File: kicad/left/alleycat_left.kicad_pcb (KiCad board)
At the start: 2 copper layers, 134 x 128 mm, 116 parts, among them J1 Conn_01x04_Male, J2 USB_C_Receptacle_USB2.0, SW1 SW_Push, SW2 RotaryEncoder_Switch, U1 nRF52840_holyiot_18010, U2 TP4056, U3 DW01A, U4 FS8205, U5 SRV05-4, U6 XC6206PxxxMR

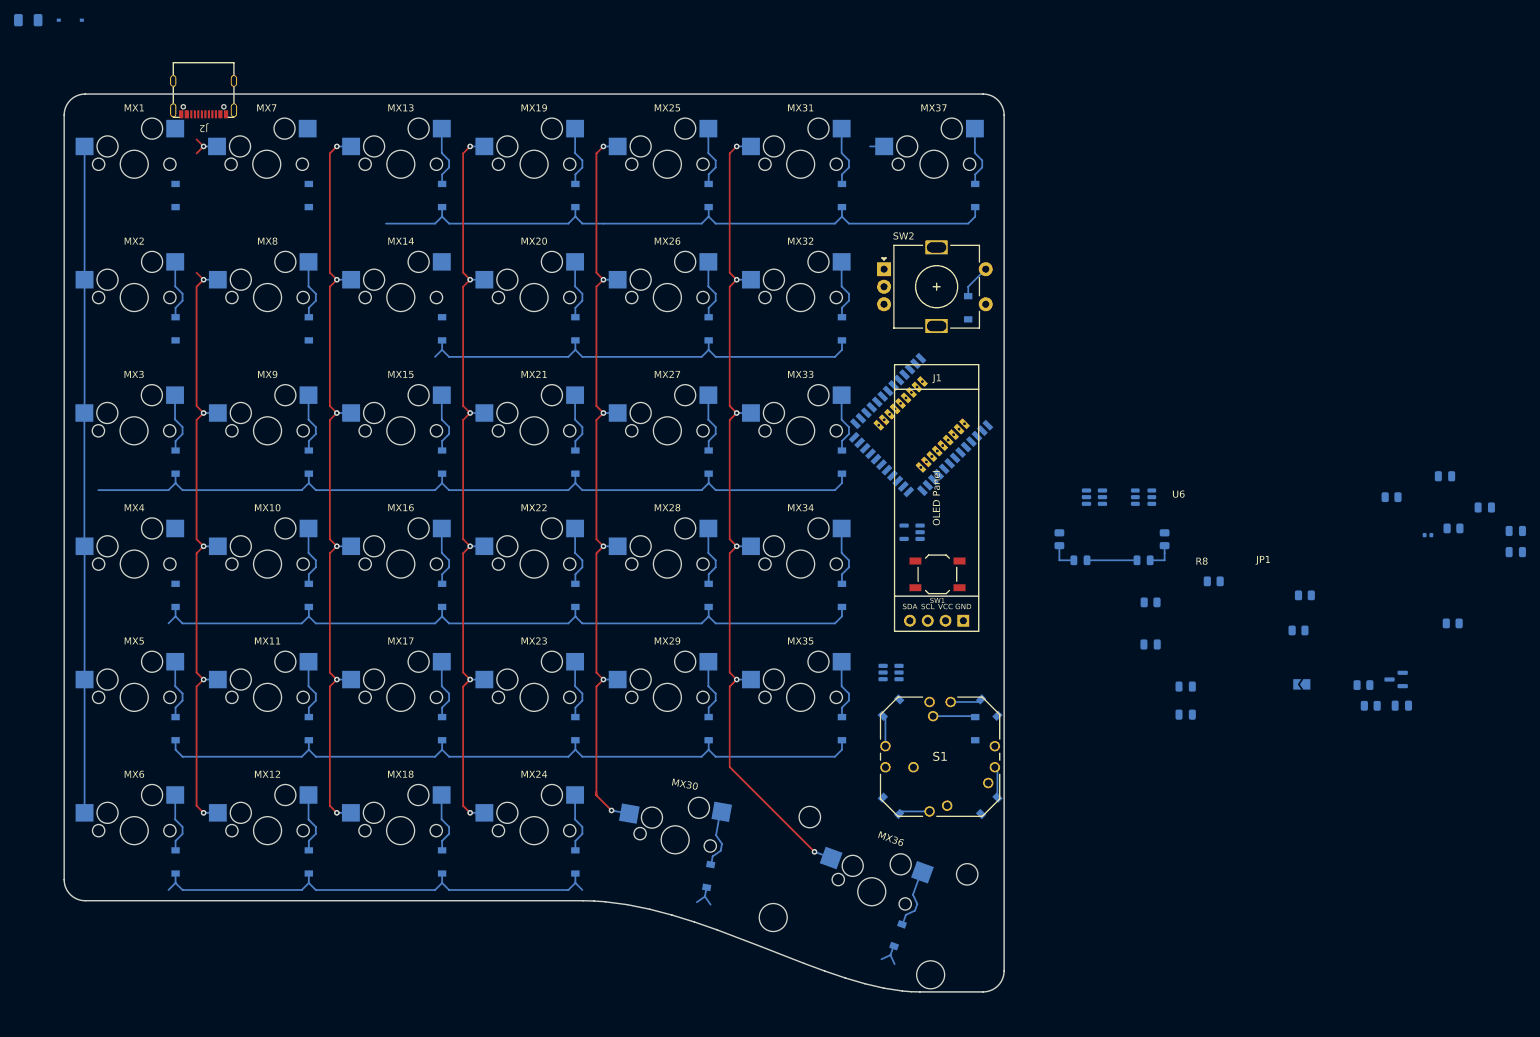
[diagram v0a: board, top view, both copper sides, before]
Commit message: pogged
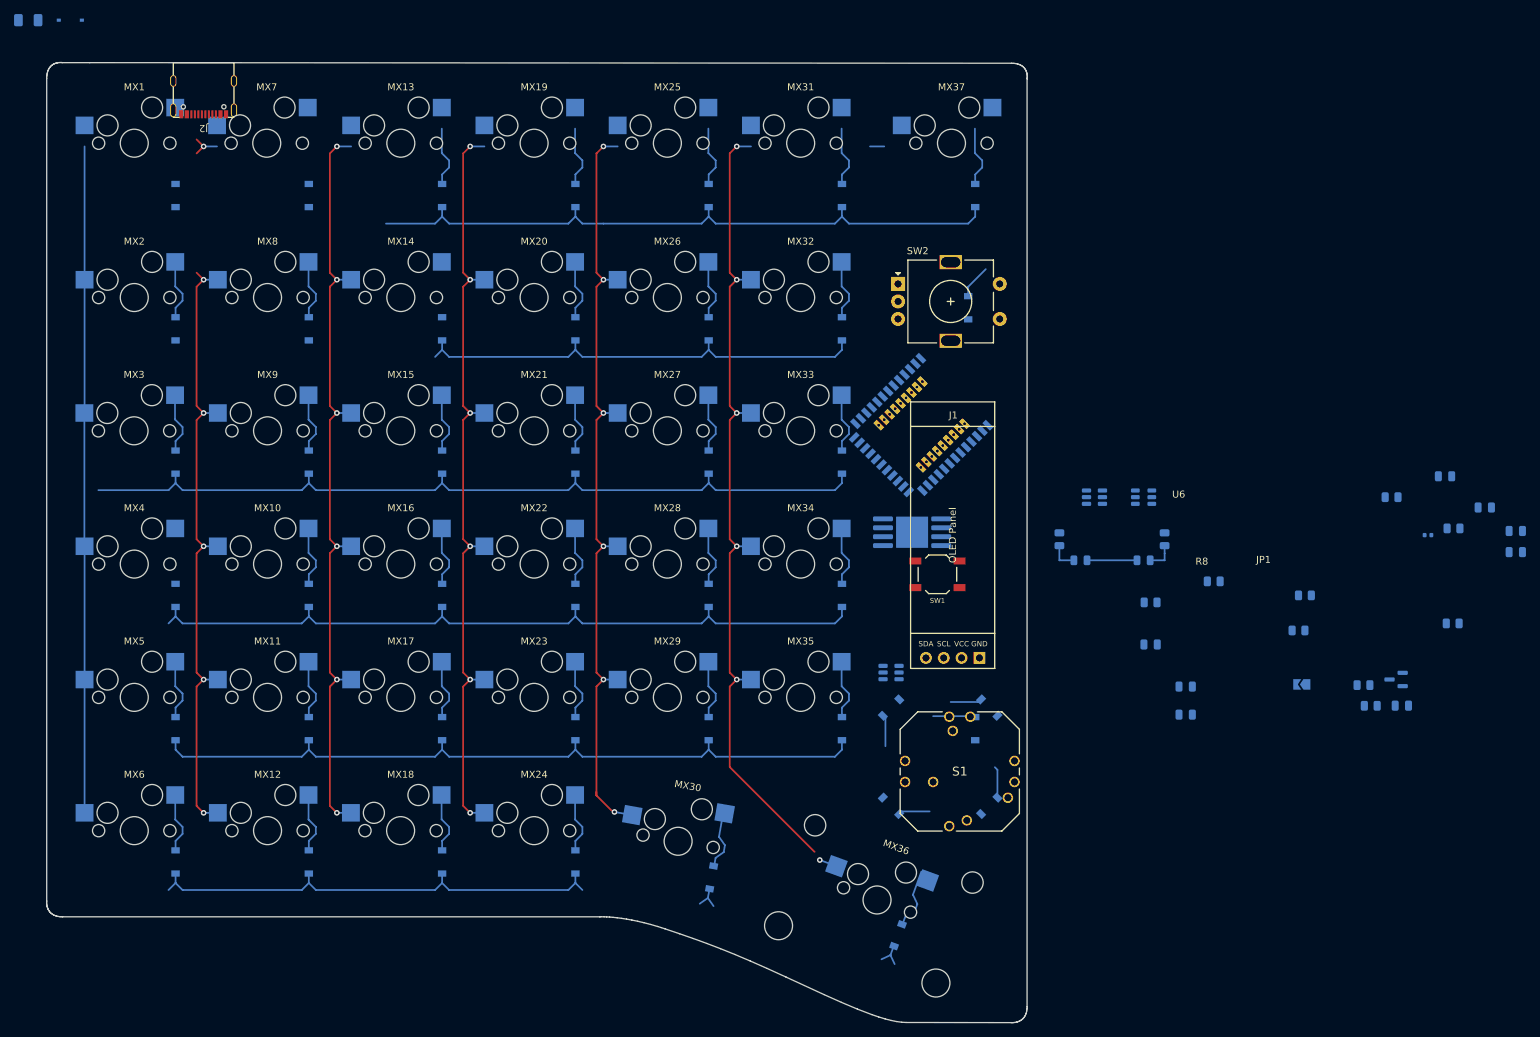
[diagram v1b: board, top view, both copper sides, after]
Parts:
- U2: footprint Package_TO_SOT_SMD:SOT-23-5 -> Package_SO:SOP-8-1EP_4.57x4.57mm_P1.27mm_EP4.57x4.45mm
- moved J1 5.77 mm to (147.8, 59.4)
- moved MX37 3.91 mm to (134.5, 20.0)
- moved S1 3.50 mm to (142.8, 112.1)
- moved MX1 3.00 mm to (18.0, 20.0)
- moved MX13 3.00 mm to (56.0, 20.0)
- moved MX19 3.00 mm to (75.0, 20.0)
- moved MX25 3.00 mm to (94.0, 20.0)
- moved MX31 3.00 mm to (113.0, 20.0)
- moved MX7 3.00 mm to (36.9, 20.0)
- moved SW2 2.90 mm to (141.5, 45.1)
- moved MX36 1.39 mm to (125.2, 125.6)
- moved D30 0.47 mm to (107.4, 127.2)
- moved MX30 0.47 mm to (96.1, 118.3)
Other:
- board size 134 x 128 mm -> 139.8 x 136.9 mm
